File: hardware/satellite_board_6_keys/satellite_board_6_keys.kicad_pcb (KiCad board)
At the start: 4 copper layers, 60.7 x 52.6 mm, 20 parts, among them J1 Conn_01x02_Socket, J2 Conn_01x06_Socket, J3 Conn_01x06_Socket, J4 Conn_02x12_Odd_Even, J5 Conn_02x12_Odd_Even, U1 CD74HCT251E, U2 CD74HCT251E

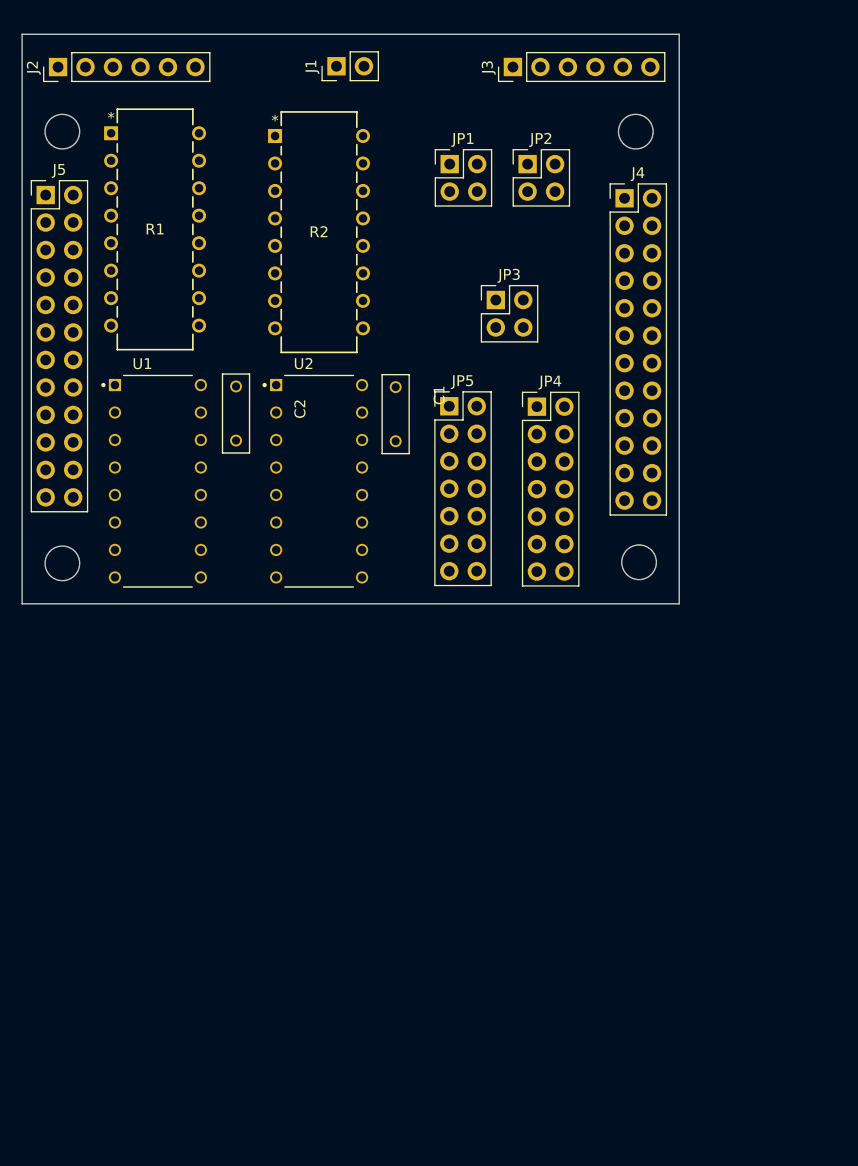
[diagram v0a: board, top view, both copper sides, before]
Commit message: First routing of the satellite board
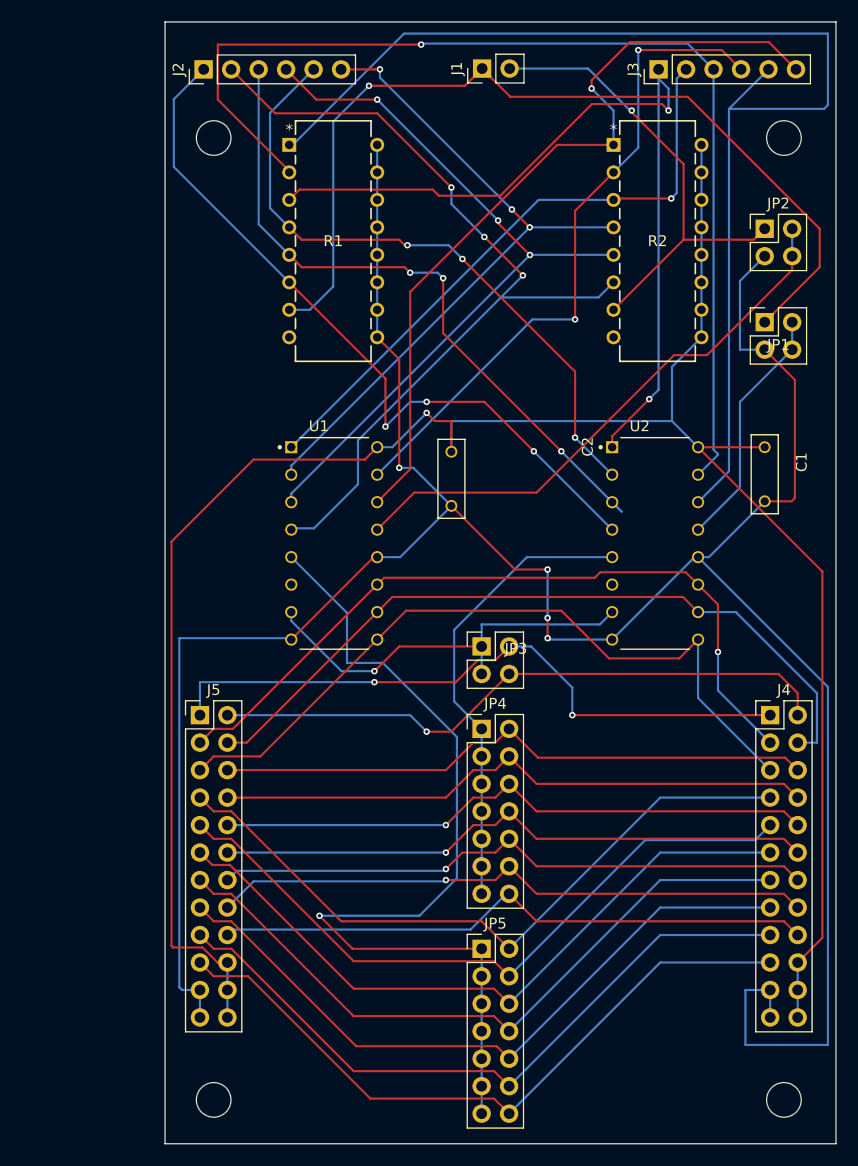
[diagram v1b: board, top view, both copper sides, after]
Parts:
- moved REF** 51.5 mm to (92.1, 137.2)
- moved REF** 51.5 mm to (144.8, 137.2)
- moved JP5 50.2 mm to (116.8, 123.2)
- moved J5 50.1 mm to (90.8, 101.6)
- moved J4 49.6 mm to (143.5, 101.6)
- moved C1 34.6 mm to (143.0, 79.3)
- moved JP1 32.6 mm to (143.0, 65.3)
- moved JP3 32.0 mm to (116.8, 95.2)
- moved U2 31.6 mm to (132.9, 85.7)
- moved R2 31.3 mm to (129.0, 48.9)
- moved JP4 30.2 mm to (116.8, 102.9)
- moved JP2 22.7 mm to (143.0, 56.6)
- moved C2 20.8 mm to (114.0, 79.8)
- moved U1 17.3 mm to (103.2, 85.7)
- moved R1 16.5 mm to (99.1, 48.9)
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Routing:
- net GND: track 0.00 -> 244.4 mm, vias 0 -> 4
- net VCC: track 0.00 -> 200.1 mm, vias 0 -> 1
- net Net-(J3-Pin_5): track 0.00 -> 112.6 mm
- net Net-(J3-Pin_3): track 0.00 -> 99.8 mm, vias 0 -> 1
- net Net-(J1-Pin_1): track 0.00 -> 84.1 mm, vias 0 -> 1
- net Net-(JP5-Pin_1): track 0.00 -> 83.6 mm, vias 0 -> 1
- net Net-(J3-Pin_1): track 0.00 -> 80.3 mm, vias 0 -> 2
- net Net-(J2-Pin_2): track 0.00 -> 80.2 mm, vias 0 -> 3
- net Net-(J3-Pin_6): track 0.00 -> 73.3 mm, vias 0 -> 1
- net Net-(J4-Pin_3): track 0.00 -> 70.4 mm, vias 0 -> 1
- net Net-(J4-Pin_4): track 0.00 -> 70.1 mm
- net Net-(J4-Pin_5): track 0.00 -> 69.5 mm
- net Net-(J2-Pin_4): track 0.00 -> 69.5 mm, vias 0 -> 3
- net Net-(J2-Pin_1): track 0.00 -> 69.1 mm, vias 0 -> 3
- net Net-(J4-Pin_19): track 0.00 -> 64.3 mm
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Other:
- board size 60.7 x 52.6 mm -> 62 x 103.7 mm
- copper layers 4 -> 2
